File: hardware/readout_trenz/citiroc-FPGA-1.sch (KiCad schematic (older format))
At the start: 17 parts

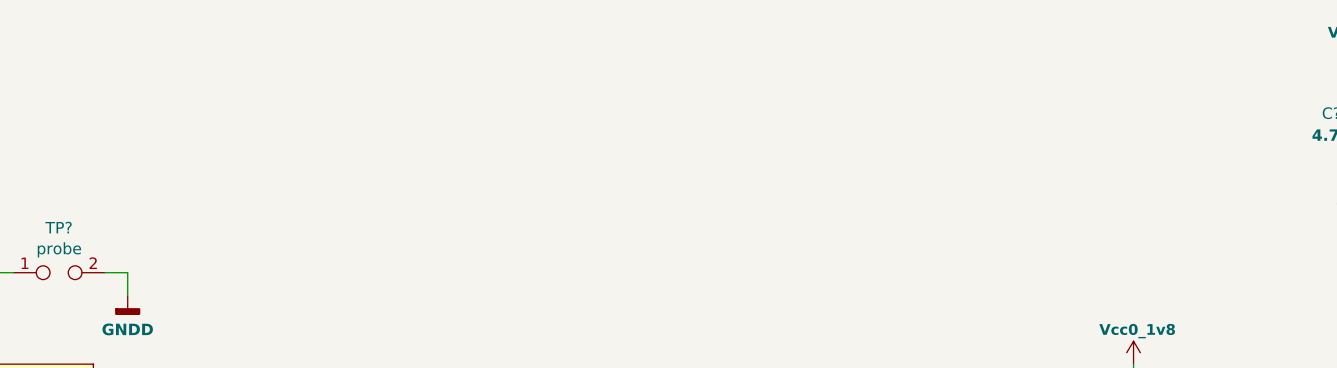
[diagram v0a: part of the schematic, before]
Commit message: Trenz Module Work in Progress
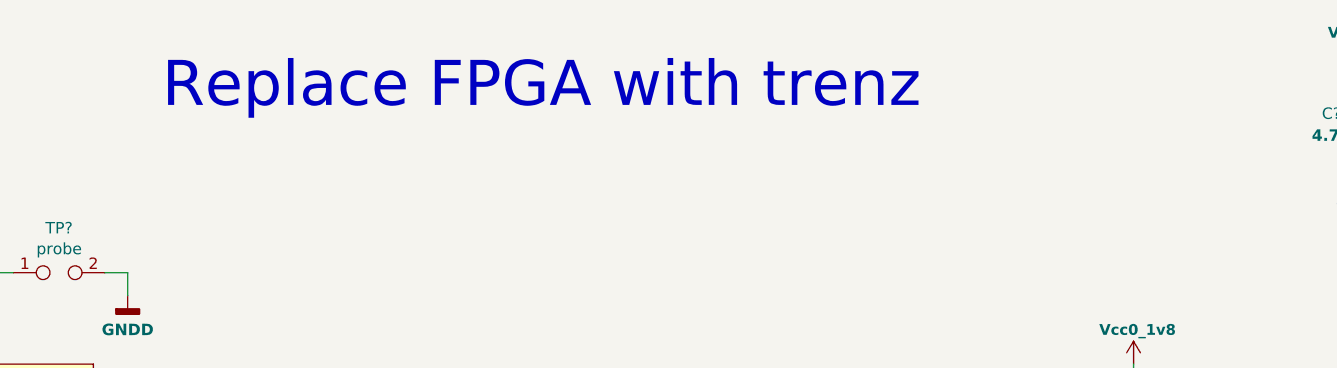
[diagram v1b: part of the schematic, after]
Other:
- note added: "Replace FPGA with trenz"
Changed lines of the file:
@@
 $Descr A4 11693 8268
 encoding utf-8
-Sheet 11 12
+Sheet 11 13
 Title ""
 Date ""
@@
 	1    0    0    -1
 $EndComp
+Text Notes 4250 1000 0    197  ~ 0
+Replace FPGA with trenz
 $EndSCHEMATC
